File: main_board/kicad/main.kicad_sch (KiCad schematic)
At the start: 1 part

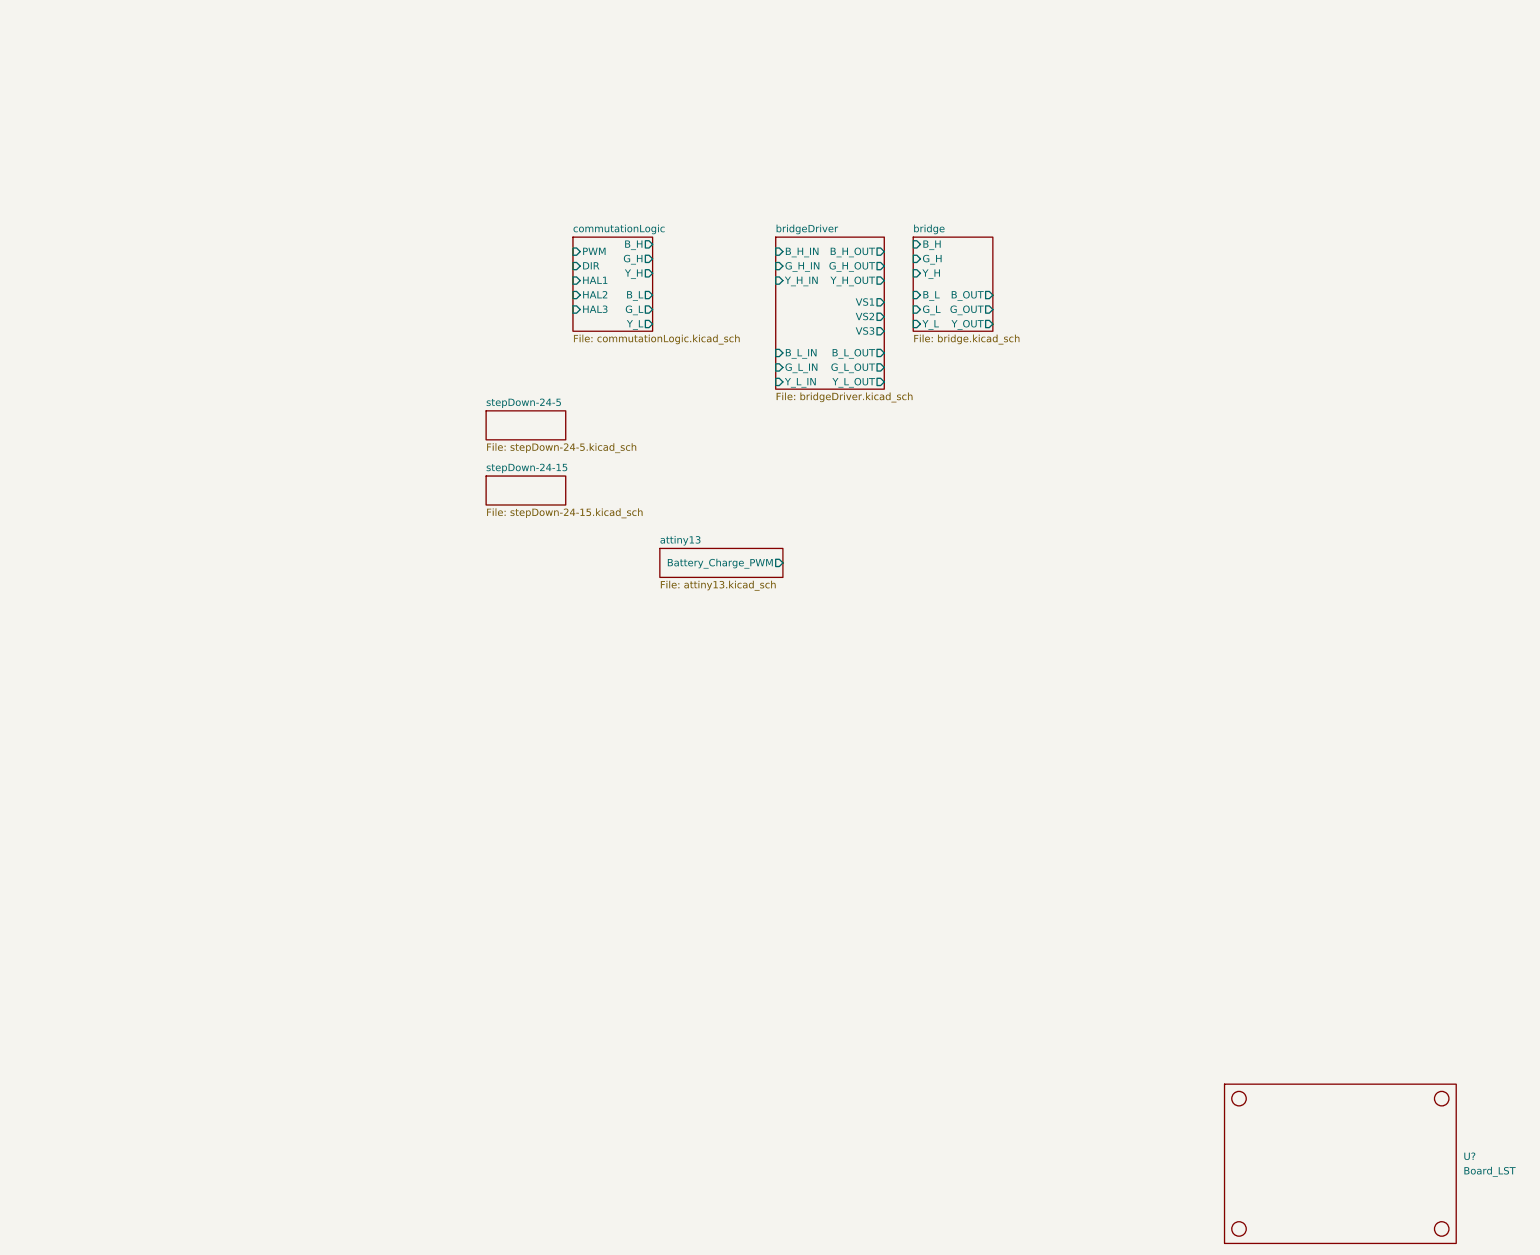
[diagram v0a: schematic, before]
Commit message: huh
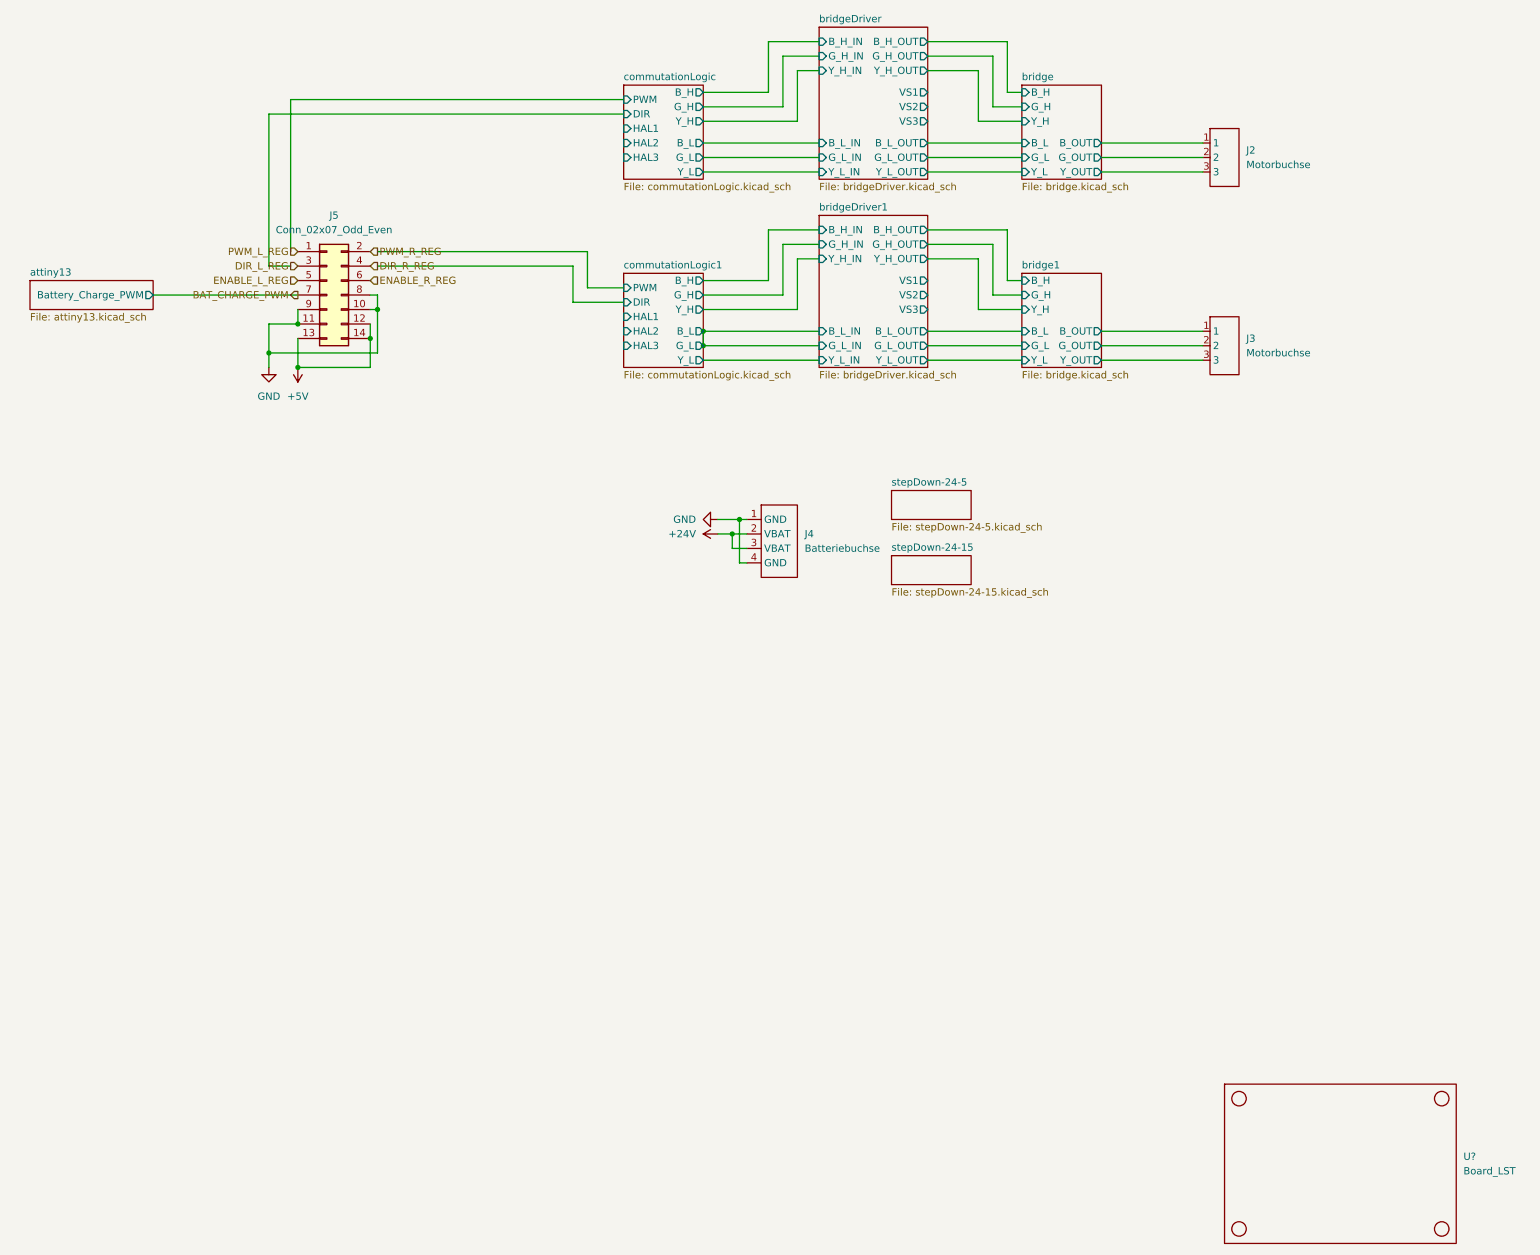
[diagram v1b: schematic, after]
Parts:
- added J2, J3: Motorbuchse, 2022-lsd:Motorbuchse, symbol 2022-lsd:Motorbuchse
- added J4: Batteriebuchse, 2022-lsd:Batteriebuchse, symbol 2022-lsd:Batteriebuchse
- added J5: Conn_02x07_Odd_Even, symbol Connector_Generic:Conn_02x07_Odd_Even
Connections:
- net bridge/B_OUT: now also J2.1
- net bridge/G_OUT: now also J2.2
- net bridge/Y_OUT: now also J2.3
- new net +24V: J4.2 (VBAT), J4.3 (VBAT)
- new net +5V: J5.12 (Pin_12), J5.13 (Pin_13), J5.14 (Pin_14)
- new net BAT_CHARGE_PWM: J5.7 (Pin_7)
- new net DIR_L_REG: J5.3 (Pin_3)
- new net DIR_R_REG: J5.4 (Pin_4)
- new net ENABLE_L_REG: J5.5 (Pin_5)
- new net ENABLE_R_REG: J5.6 (Pin_6)
- new net GND: J4.1 (GND), J4.4 (GND), J5.10 (Pin_10), J5.11 (Pin_11), J5.8 (Pin_8), J5.9 (Pin_9)
- new net PWM_L_REG: J5.1 (Pin_1)
- new net PWM_R_REG: J5.2 (Pin_2)
- new net bridge1/B_OUT: J3.1
- new net bridge1/G_OUT: J3.2
- new net bridge1/Y_OUT: J3.3
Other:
- added sheet bridge1 (bridge.kicad_sch)
- added sheet bridgeDriver1 (bridgeDriver.kicad_sch)
- added sheet commutationLogic1 (commutationLogic.kicad_sch)
